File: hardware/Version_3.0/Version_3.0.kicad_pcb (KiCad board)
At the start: 2 copper layers, 21.4 x 21 mm, 44 parts, among them J1 Conn_02x05_Counter_Clockwise, J2 Conn_Coaxial, U1 ADF4351, Y1 SG-5032CAN

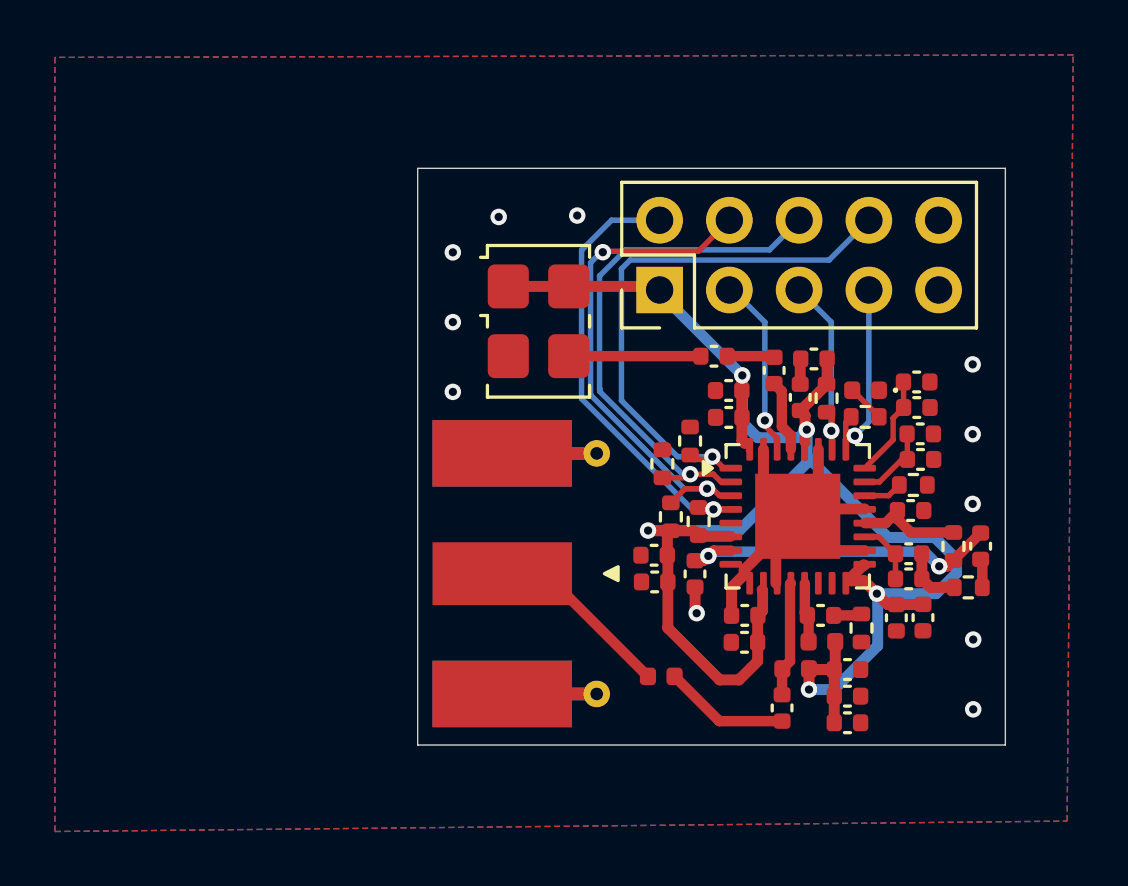
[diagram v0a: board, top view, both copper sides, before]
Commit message: updated pcb to 4 layers and the images. this is for v3
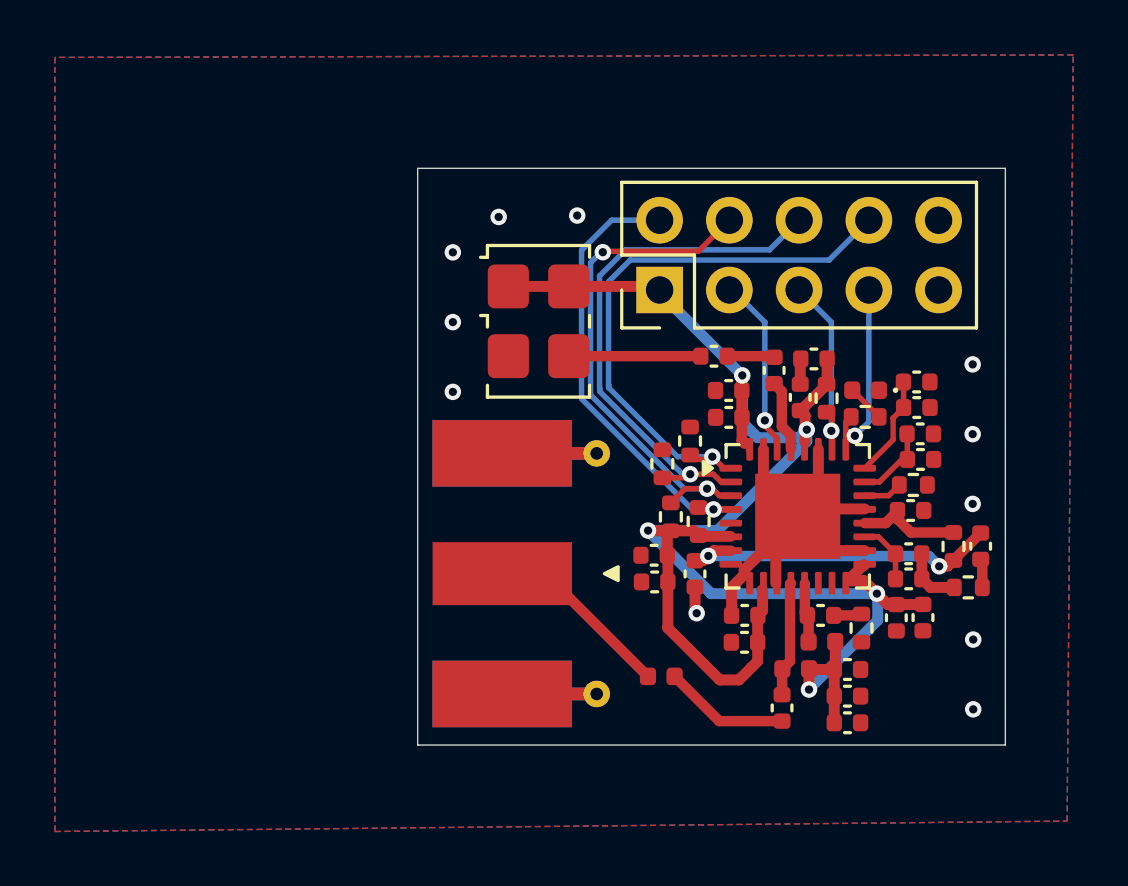
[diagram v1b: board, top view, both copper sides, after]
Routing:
- net +3.3V: track 67.4 -> 64.0 mm
- added copper zone on In1.Cu, net GND
- added copper zone on In2.Cu, net GND
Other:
- copper layers 2 -> 4
